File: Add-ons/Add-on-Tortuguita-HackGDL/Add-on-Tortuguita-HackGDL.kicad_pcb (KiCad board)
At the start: 2 copper layers, 50 x 38.9 mm, 0 parts

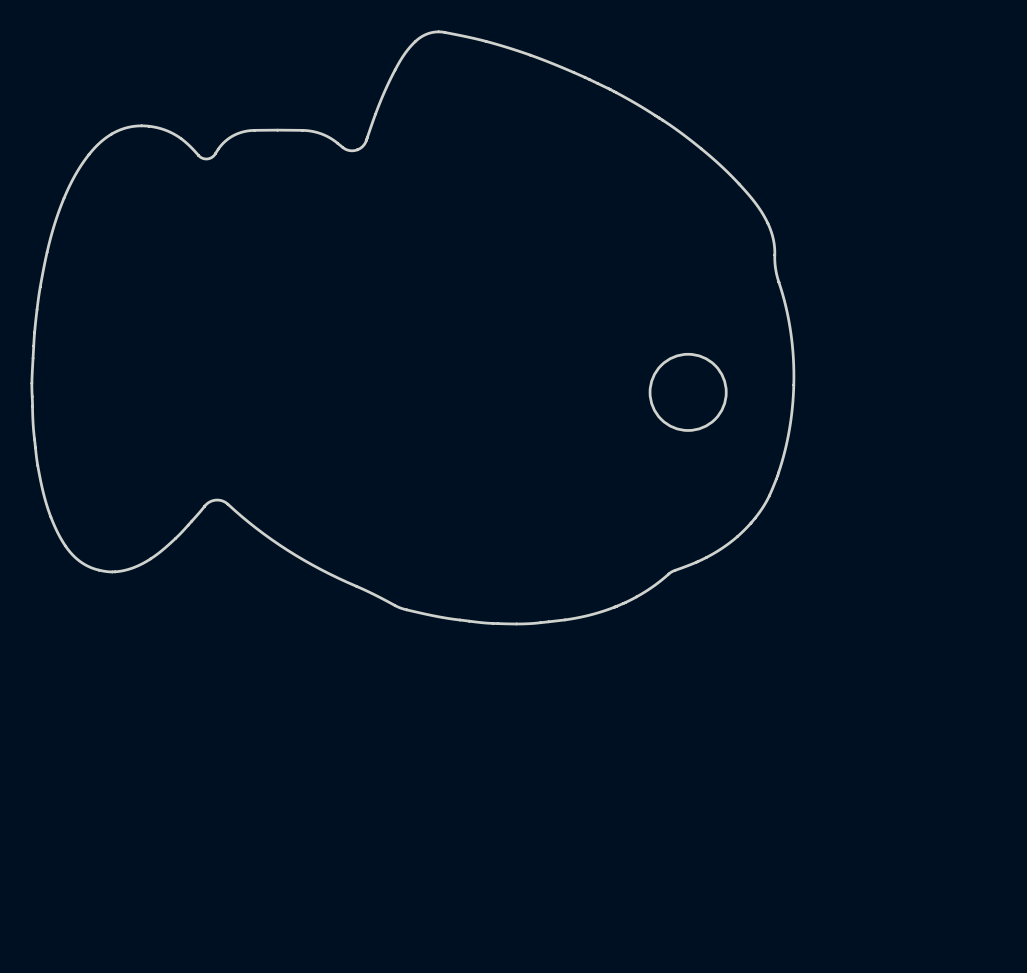
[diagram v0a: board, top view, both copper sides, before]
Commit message: feat(Hw):Update_Route_And_Init_Addon_Tortuguita
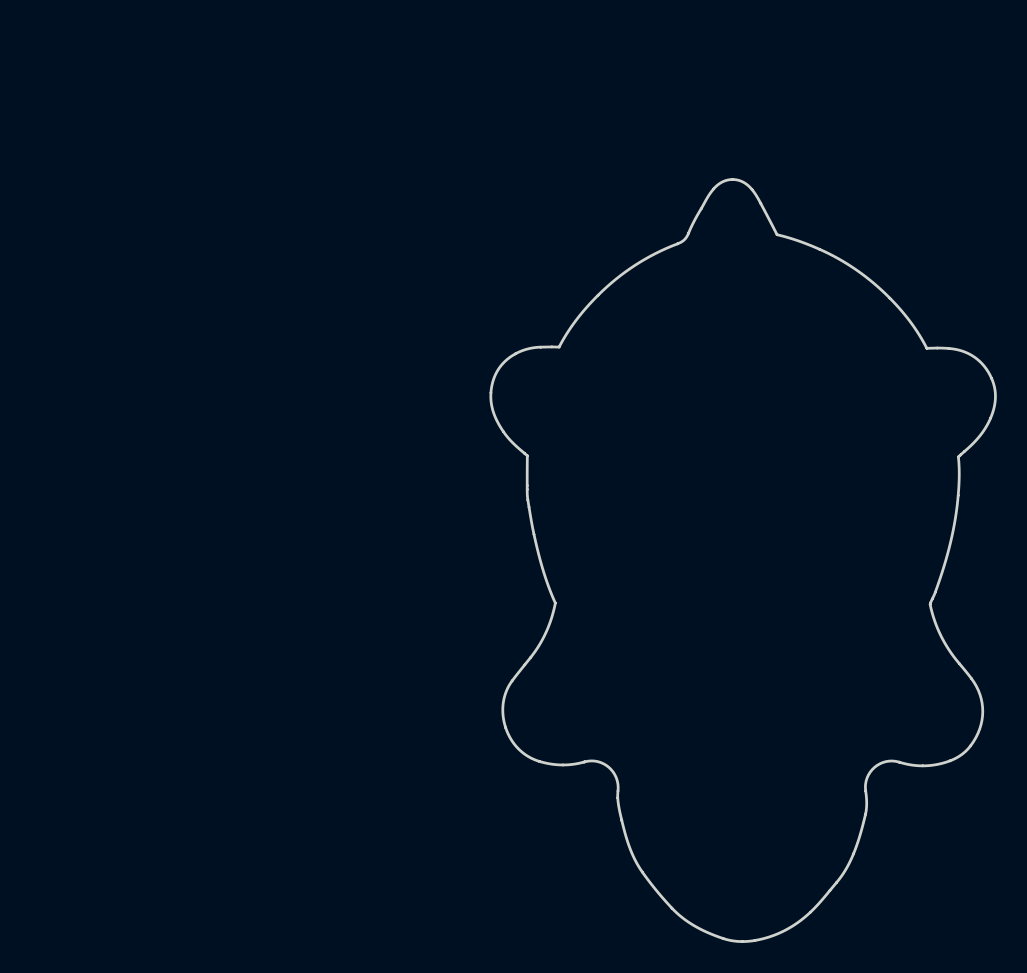
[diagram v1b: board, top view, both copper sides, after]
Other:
- board size 50 x 38.9 mm -> 33.1 x 50 mm
